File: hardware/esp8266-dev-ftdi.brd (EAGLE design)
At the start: 50 x 50 mm, 63 parts, among them CON1 USBMICRO-NO_CENTER-LONG_PADS

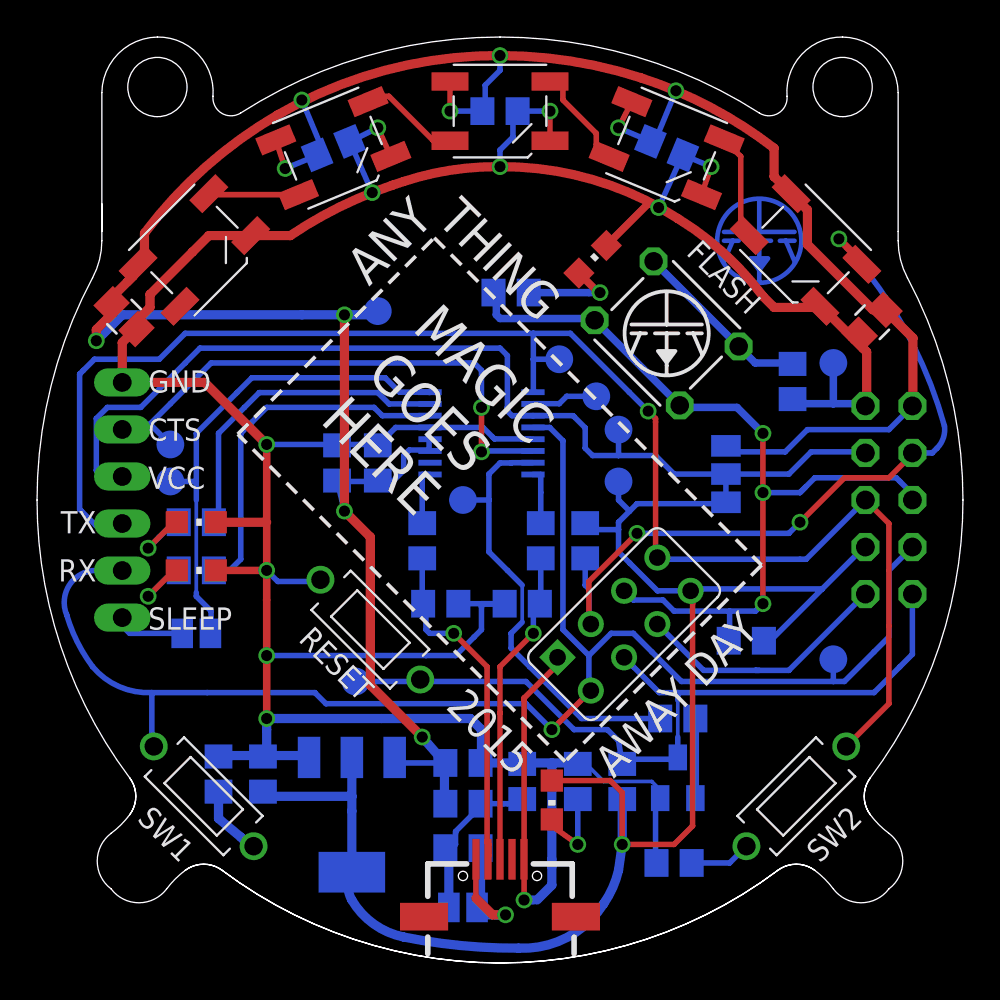
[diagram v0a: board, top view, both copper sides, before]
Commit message: cosmetics
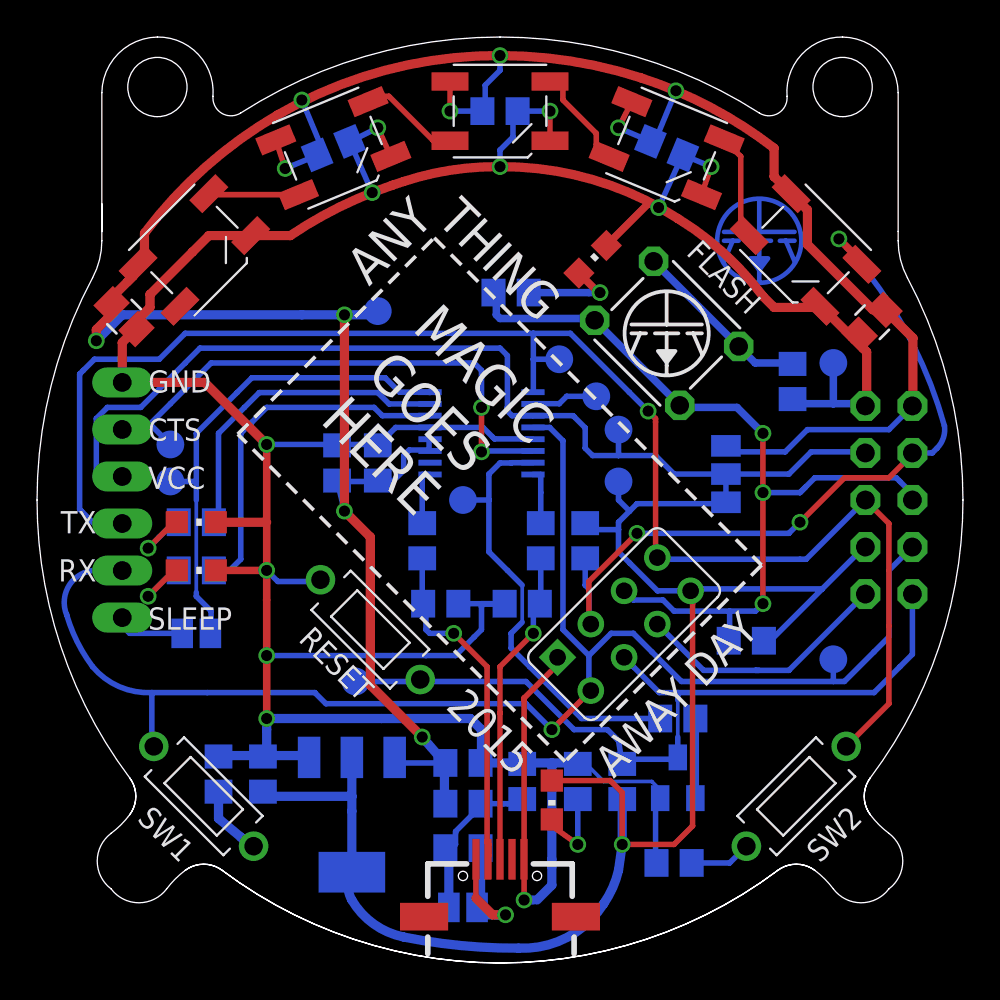
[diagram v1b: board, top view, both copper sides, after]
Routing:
- net VCCIO: track 56.8 -> 55.2 mm
- net +3V3: track 89.1 -> 90.3 mm
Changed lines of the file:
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@@
 <setting verticaltext="up"/>
 </settings>
-<grid distance="1" unitdist="mm" unit="mm" style="lines" multiple="1" display="yes" altdistance="0.1" altunitdist="mm" altunit="mm"/>
+<grid distance="0.1" unitdist="mm" unit="mm" style="lines" multiple="1" display="yes" altdistance="0.05" altunitdist="mm" altunit="mm"/>
 <layers>
-<layer number="1" name="Top" color="4" fill="1" visible="no" active="yes"/>
+<layer number="1" name="Top" color="4" fill="1" visible="yes" active="yes"/>
 <layer number="16" name="Bottom" color="1" fill="1" visible="no" active="yes"/>
-<layer number="17" name="Pads" color="2" fill="1" visible="no" active="yes"/>
-<layer number="18" name="Vias" color="2" fill="1" visible="no" active="yes"/>
-<layer number="19" name="Unrouted" color="6" fill="1" visible="no" active="yes"/>
-<layer number="20" name="Dimension" color="15" fill="1" visible="no" active="yes"/>
-<layer number="21" name="tPlace" color="7" fill="1" visible="no" active="yes"/>
+<layer number="17" name="Pads" color="2" fill="1" visible="yes" active="yes"/>
+<layer number="18" name="Vias" color="2" fill="1" visible="yes" active="yes"/>
+<layer number="19" name="Unrouted" color="6" fill="1" visible="yes" active="yes"/>
+<layer number="20" name="Dimension" color="15" fill="1" visible="yes" active="yes"/>
+<layer number="21" name="tPlace" color="7" fill="1" visible="yes" active="yes"/>
 <layer number="22" name="bPlace" color="7" fill="1" visible="no" active="yes"/>
-<layer number="23" name="tOrigins" color="15" fill="1" visible="no" active="yes"/>
+<layer number="23" name="tOrigins" color="15" fill="1" visible="yes" active="yes"/>
 <layer number="24" name="bOrigins" color="15" fill="1" visible="no" active="yes"/>
-<layer number="25" name="tNames" color="7" fill="1" visible="no" active="yes"/>
+<layer number="25" name="tNames" color="7" fill="1" visible="yes" active="yes"/>
 <layer number="26" name="bNames" color="7" fill="1" visible="no" active="yes"/>
 <layer number="27" name="tValues" color="7" fill="1" visible="yes" active="yes"/>
-<layer number="28" name="bValues" color="7" fill="1" visible="yes" active="yes"/>
-<layer number="29" name="tStop" color="7" fill="3" visible="no" active="yes"/>
+<layer number="28" name="bValues" color="7" fill="1" visible="no" active="yes"/>
+<layer number="29" name="tStop" color="7" fill="3" visible="yes" active="yes"/>
 <layer number="30" name="bStop" color="7" fill="6" visible="no" active="yes"/>
 <layer number="31" name="tCream" color="7" fill="4" visible="no" active="yes"/>
@@
 <text x="43.2" y="22" size="1.2" layer="22" font="vector" ratio="15" rot="MR270" align="bottom-center">3V3</text>
 <text x="44.8" y="18.6" size="1.2" layer="22" font="vector" ratio="15" rot="MR270" align="center-left">16</text>
-<text x="48.4" y="27.6" size="1.2" layer="22" font="vector" ratio="15" rot="MR270" align="top-center">2</text>
-<text x="48.4" y="25" size="1.2" layer="22" font="vector" ratio="15" rot="MR270" align="top-center">0</text>
-<text x="48.4" y="22.4" size="1.2" layer="22" font="vector" ratio="15" rot="MR270" align="top-center">RX</text>
+<text x="48.4" y="27.6" size="1" layer="22" font="vector" ratio="15" rot="MR270" align="top-center">2</text>
+<text x="48.4" y="25" size="1" layer="22" font="vector" ratio="15" rot="MR270" align="top-center">0</text>
+<text x="48.4" y="22.7" size="1" layer="22" font="vector" ratio="15" rot="MR270" align="top-center">RX</text>
 <text x="47.2" y="18.8" size="1.2" layer="22" font="vector" ratio="15" rot="MR270" align="center-left">RES</text>
 <text x="17.6" y="36" size="1.7" layer="22" font="vector" ratio="15" rot="MR0">ESP 8266
@@
 </class>
 </classes>
-<designrules name="Elecrow_2-layer_eagle_rule *">
-<description language="de">&lt;b&gt;EAGLE Design Rules&lt;/b&gt;
-&lt;p&gt;
-Die Standard-Design-Rules sind so gewählt, dass sie für
-die meisten Anwendungen passen. Sollte ihre Platine
-besondere Anforderungen haben, treffen Sie die erforderlichen
-Einstellungen hier und speichern die Design Rules unter
-einem neuen Namen ab.</description>
-<description language="en">&lt;b&gt;EAGLE Design Rules&lt;/b&gt;
-&lt;p&gt;
-The default Design Rules have been set to cover
-a wide range of applications. Your particular design
-may have different requirements, so please make the
-necessary adjustments and save your customized
-design rules under a new name.</description>
-<description language="zh">&lt;b&gt;Elecrow EAGLE Design Rules&lt;/b&gt;
-</description>
+<designrules name="dirt_cheap_dirty_boards.v1 *">
+<description language="en">&lt;b&gt;Dirty Cheap Dirty Board Design Rules&lt;/b&gt;
+&lt;br&gt;
+&lt;br&gt;Min width/Spacing: 5/5mil
+&lt;br&gt;Min diameter of finished hole 12mil</description>
 <param name="layerSetup" value="(1*16)"/>
-<param name="mtCopper" value="0.035mm 0.035mm 0.035mm 0.035mm 0.035mm 0.035mm 0.035mm 0.035mm 0.035mm 0.035mm 0.035mm 0.035mm 0.035mm 0.035mm 0.035mm 0.035mm"/>
-<param name="mtIsolate" value="1.5mm 0.15mm 0.2mm 0.15mm 0.2mm 0.15mm 0.2mm 0.15mm 0.2mm 0.15mm 0.2mm 0.15mm 0.2mm 0.15mm 0.2mm"/>
-<param name="mdWireWire" value="6mil"/>
-<param name="mdWirePad" value="6mil"/>
-<param name="mdWireVia" value="6mil"/>
-<param name="mdPadPad" value="6mil"/>
-<param name="mdPadVia" value="6mil"/>
-<param name="mdViaVia" value="6mil"/>
+<param name="mtCopper" value="0.035mm 0.0175mm 0.035mm 0.035mm 0.035mm 0.035mm 0.035mm 0.035mm 0.035mm 0.035mm 0.035mm 0.035mm 0.035mm 0.035mm 0.0175mm 0.035mm"/>
+<param name="mtIsolate" value="1.5mm 1.1mm 0.2mm 0.15mm 0.2mm 0.15mm 0.2mm 0.15mm 0.2mm 0.15mm 0.2mm 0.15mm 0.2mm 0.15mm 0.2mm"/>
+<param name="mdWireWire" value="5mil"/>
+<param name="mdWirePad" value="5mil"/>
+<param name="mdWireVia" value="5mil"/>
+<param name="mdPadPad" value="5mil"/>
+<param name="mdPadVia" value="5mil"/>
+<param name="mdViaVia" value="5mil"/>
 <param name="mdSmdPad" value="0mil"/>
 <param name="mdSmdVia" value="0mil"/>
@@
 <param name="mdDrill" value="10mil"/>
 <param name="mdSmdStop" value="0mil"/>
-<param name="msWidth" value="6mil"/>
+<param name="msWidth" value="5mil"/>
 <param name="msDrill" value="12mil"/>
 <param name="msMicroVia" value="12mil"/>
 <param name="msBlindViaRatio" value="0.5"/>
-<param name="rvPadTop" value="0.25"/>
-<param name="rvPadInner" value="0.25"/>
-<param name="rvPadBottom" value="0.25"/>
+<param name="rvPadTop" value="0.3"/>
+<param name="rvPadInner" value="0.3"/>
+<param name="rvPadBottom" value="0.3"/>
 <param name="rvViaOuter" value="0.25"/>
 <param name="rvViaInner" value="0.25"/>
@@
 <param name="rvMicroViaInner" value="0.25"/>
 <param name="rlMinPadTop" value="10mil"/>
-<param name="rlMaxPadTop" value="20mil"/>
+<param name="rlMaxPadTop" value="30mil"/>
 <param name="rlMinPadInner" value="10mil"/>
-<param name="rlMaxPadInner" value="20mil"/>
+<param name="rlMaxPadInner" value="30mil"/>
 <param name="rlMinPadBottom" value="10mil"/>
-<param name="rlMaxPadBottom" value="20mil"/>
+<param name="rlMaxPadBottom" value="30mil"/>
 <param name="rlMinViaOuter" value="6mil"/>
 <param name="rlMaxViaOuter" value="20mil"/>
@@
 <param name="mlMinCreamFrame" value="0mil"/>
 <param name="mlMaxCreamFrame" value="0mil"/>
-<param name="mlViaStopLimit" value="100mil"/>
+<param name="mlViaStopLimit" value="25mil"/>
 <param name="srRoundness" value="0"/>
 <param name="srMinRoundness" value="0mil"/>
@@
 <wire x1="32" y1="21.6" x2="31.4" y2="22.2" width="0.3" layer="16"/>
 <wire x1="29.55" y1="23.4" x2="29.6" y2="23.75" width="0.3" layer="16"/>
-<wire x1="37.124" y1="24.8" x2="37.2" y2="24.876" width="0.3" layer="16"/>
 <wire x1="42.4" y1="20.2" x2="35.39605" y2="20.2" width="0.3" layer="16"/>
 <wire x1="35.39605" y1="20.2" x2="35.2921" y2="20.09605" width="0.3" layer="16"/>
@@
 <wire x1="42.4" y1="20.2" x2="39.6" y2="17.4" width="0.3" layer="16"/>
 <wire x1="39.6" y1="17.4" x2="39.25" y2="17.4" width="0.3" layer="16"/>
+<wire x1="37.124" y1="24.8" x2="37.2" y2="24.9" width="0.3" layer="16"/>
+<wire x1="37.2" y1="24.9" x2="37.2" y2="26.1" width="0.3" layer="16"/>
 </signal>
 <signal name="N$9">
@@
 <wire x1="29" y1="29.5" x2="28.947" y2="29.553" width="0.3" layer="16"/>
 <wire x1="28.947" y1="29.553" x2="26.779" y2="29.553" width="0.3" layer="16"/>
-<wire x1="37.2" y1="24.8" x2="37.2" y2="26.4" width="0.3" layer="16"/>
 <contactref element="VCC" pad="TP"/>
 <wire x1="31.4" y1="28.8" x2="31.4" y2="27.4" width="0.3" layer="16"/>
